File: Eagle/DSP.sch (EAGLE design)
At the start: 23 parts

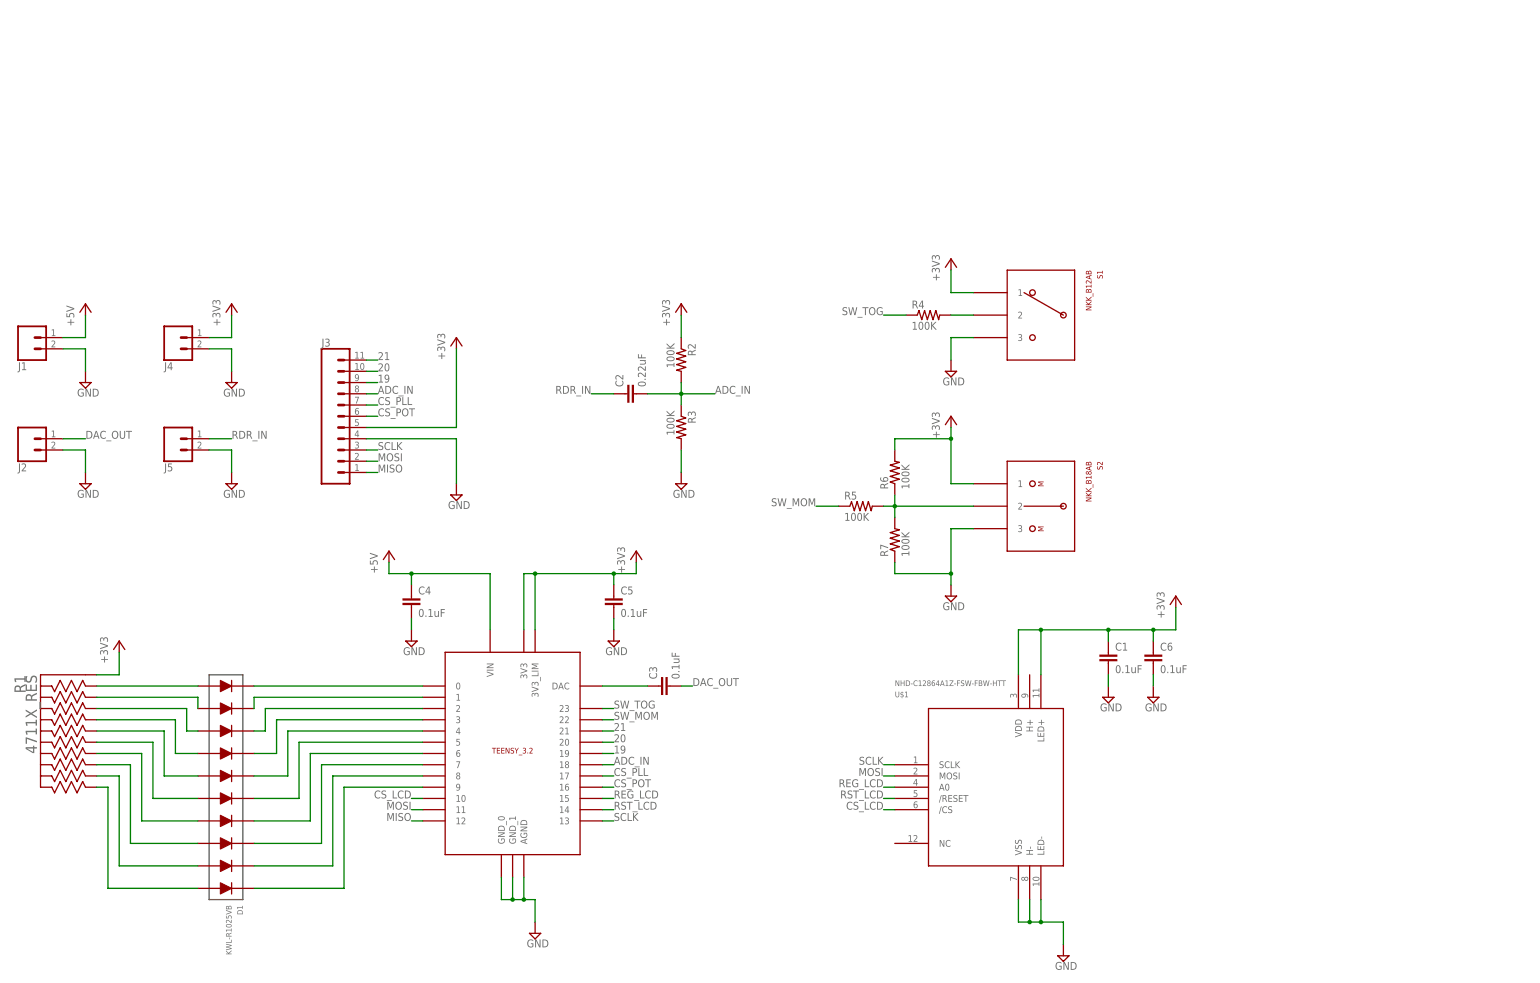
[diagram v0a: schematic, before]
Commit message: updates to dsp layout
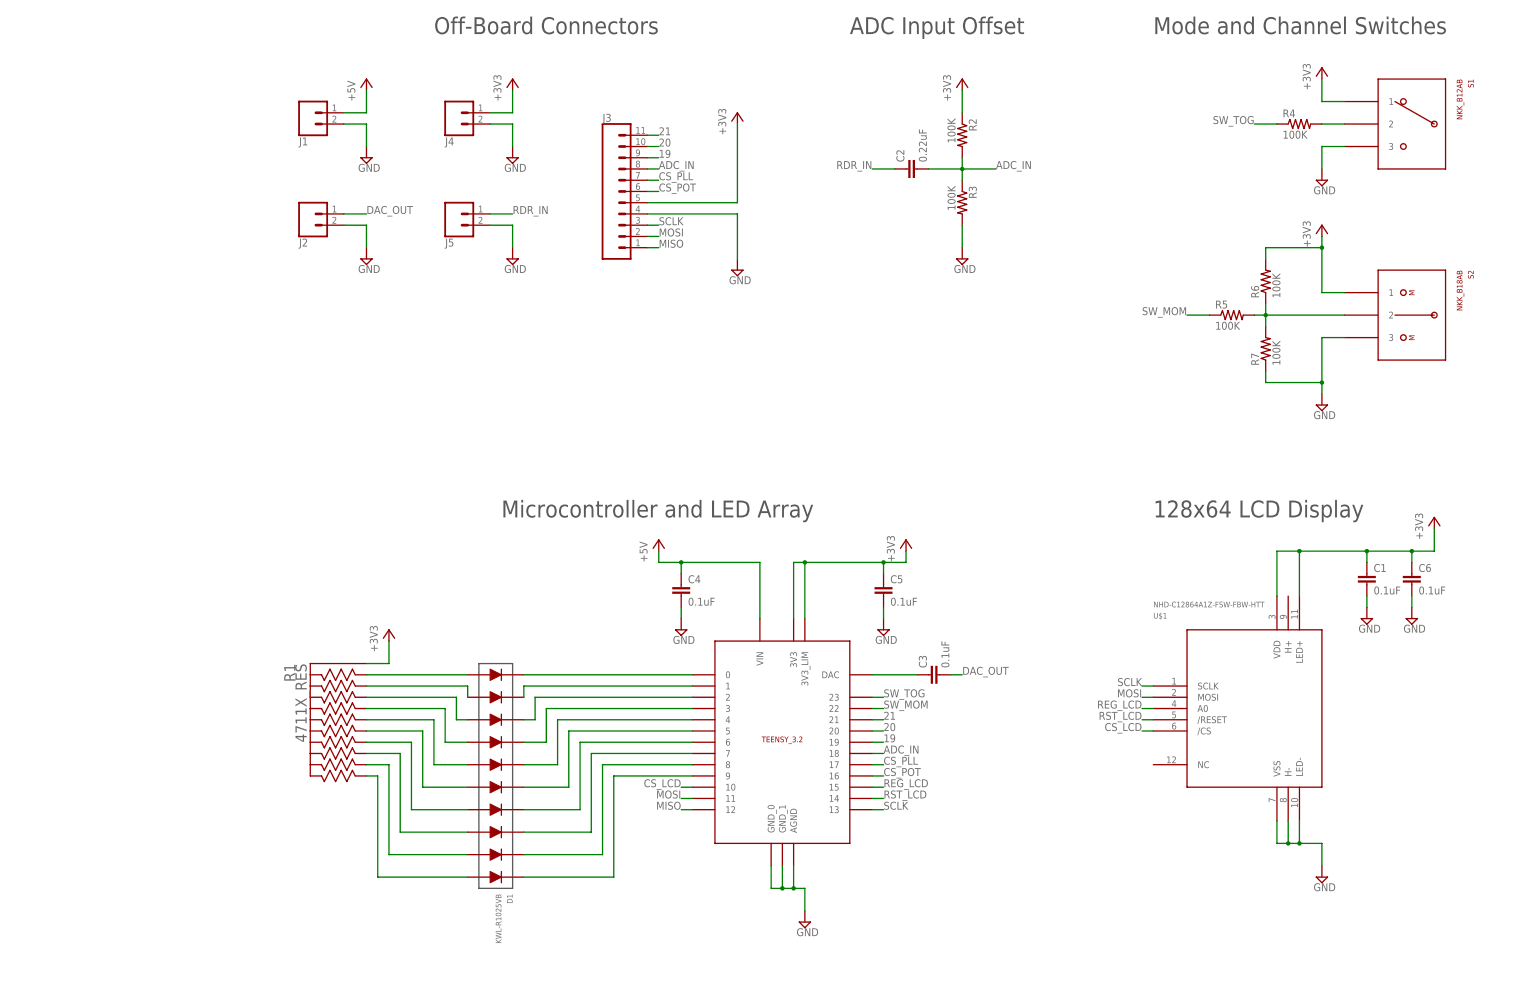
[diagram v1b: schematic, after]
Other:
- note added: "128x64 LCD Display"
- note added: "ADC Input Offset"
- note added: "Microcontroller and LED Array"
- note added: "Mode and Channel Switches"
- note added: "Off-Board Connectors"
- moved on the sheet: C1, C2, C3, C4, C5, C6, D1, J1, J2, J3, J4, J5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
